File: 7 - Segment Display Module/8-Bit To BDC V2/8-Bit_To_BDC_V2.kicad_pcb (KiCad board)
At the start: 2 copper layers, 93 x 83 mm, 42 parts, among them J1 Conn_01x08_Pin, J2 Conn_01x02_Pin, U1 AT28C64B-15PU, U2 AT28C64B-15PU, U3 4056, U4 4056, U5 4056

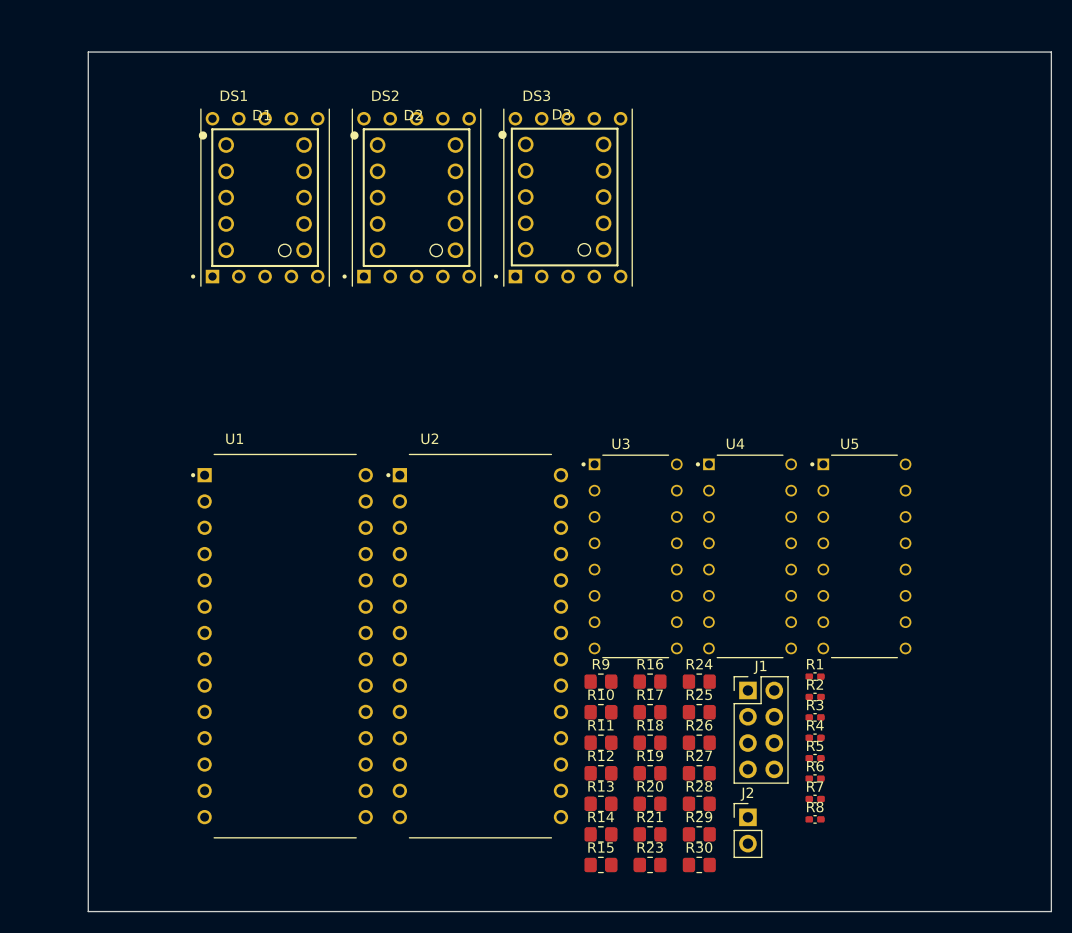
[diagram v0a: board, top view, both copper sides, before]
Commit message: PCB Layout modification
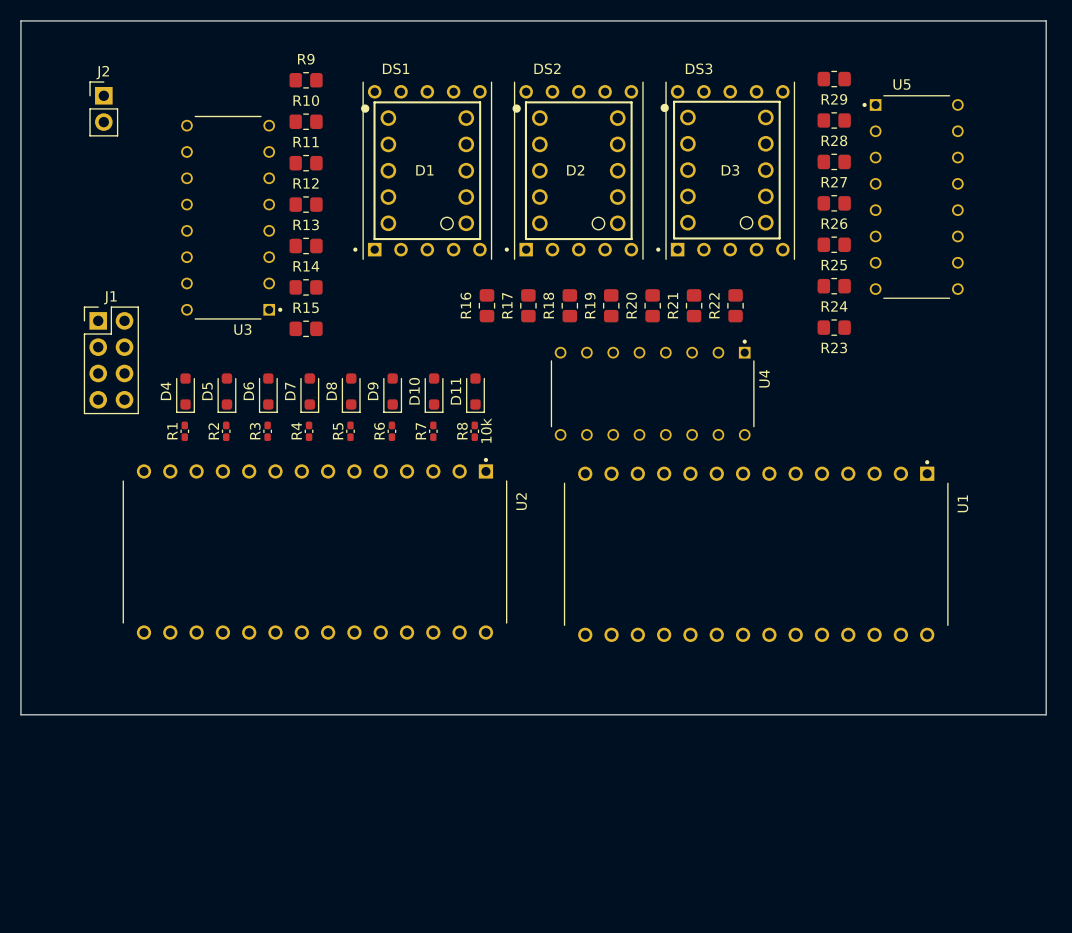
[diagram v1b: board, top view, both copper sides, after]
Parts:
- removed R30: 330, Resistor_SMD:R_0805_2012Metric_Pad1.20x1.40mm_HandSolder
- added D10: US1M, Diode_SMD:D_SOD-323_HandSoldering, F.Cu at (82.4, 60.3)
- added D11: US1M, Diode_SMD:D_SOD-323_HandSoldering, F.Cu at (86.4, 60.3)
- added D4: US1M, Diode_SMD:D_SOD-323_HandSoldering, F.Cu at (58.4, 60.3)
- added D5: US1M, Diode_SMD:D_SOD-323_HandSoldering, F.Cu at (62.4, 60.3)
- added D6: US1M, Diode_SMD:D_SOD-323_HandSoldering, F.Cu at (66.4, 60.3)
- added D7: US1M, Diode_SMD:D_SOD-323_HandSoldering, F.Cu at (70.4, 60.3)
- added D8: US1M, Diode_SMD:D_SOD-323_HandSoldering, F.Cu at (74.4, 60.3)
- added D9: US1M, Diode_SMD:D_SOD-323_HandSoldering, F.Cu at (78.4, 60.3)
- added R22: 330, Resistor_SMD:R_0805_2012Metric_Pad1.20x1.40mm_HandSolder, F.Cu at (111.5, 52.0)
- moved J2 93.4 mm to (50.5, 31.7)
- moved R29 74.1 mm to (121.0, 30.1), turned to 180 degrees
- moved J1 72.2 mm to (50.0, 53.5)
- moved R28 67.3 mm to (121.0, 34.1), turned to 180 degrees
- moved R1 65.3 mm to (58.3, 64.1), turned to 90 degrees
- moved R9 64.7 mm to (70.0, 30.2)
- moved R10 63.7 mm to (70.0, 34.2)
- moved R11 62.8 mm to (70.0, 38.2)
- moved R2 62.4 mm to (62.3, 64.1), turned to 90 degrees
- moved R12 61.9 mm to (70.0, 42.2)
- moved R13 60.9 mm to (70.0, 46.2)
- moved R27 60.5 mm to (121.0, 38.1), turned to 180 degrees
- moved R14 60.0 mm to (70.0, 50.2)
- moved R3 59.6 mm to (66.3, 64.1), turned to 90 degrees
- moved R15 59.1 mm to (70.0, 54.2)
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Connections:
- J1 pad 1: 1 -> Net-(D4-A)
- J1 pad 2: 2 -> Net-(D5-A)
- J1 pad 3: 3 -> Net-(D6-A)
- J1 pad 4: 4 -> Net-(D7-A)
- J1 pad 5: 5 -> Net-(D8-A)
- J1 pad 6: 6 -> Net-(D9-A)
- J1 pad 7: 7 -> Net-(D10-A)
- J1 pad 8: 8 -> Net-(D11-A)
- R11 pad 1: Net-(U3-a) -> Net-(U3-c)
- R11 pad 2: H-A -> H-C
- R23 pad 1: Net-(U4-g) -> Net-(U5-a)
- R23 pad 2: T-G -> O-A
- R24 pad 1: Net-(U5-a) -> Net-(U5-b)
- R24 pad 2: O-A -> O-B
- R25 pad 1: Net-(U5-b) -> Net-(U5-c)
- R25 pad 2: O-B -> O-C
- R26 pad 1: Net-(U5-c) -> Net-(U5-d)
- R26 pad 2: O-C -> O-D
- R27 pad 1: Net-(U5-d) -> Net-(U5-e)
- R27 pad 2: O-D -> O-E
- R28 pad 1: Net-(U5-e) -> Net-(U5-f)
- R28 pad 2: O-E -> O-F
- R29 pad 1: Net-(U5-f) -> Net-(U5-g)
- R29 pad 2: O-F -> O-G
- R9 pad 1: Net-(U3-c) -> Net-(U3-a)
- R9 pad 2: H-C -> H-A
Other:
- board size 93 x 83 mm -> 99 x 67 mm
